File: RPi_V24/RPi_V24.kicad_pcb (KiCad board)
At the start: 4 copper layers, 65 x 56 mm, 65 parts, among them J1 DB9_Male, J10 Conn_01x03, J11 Conn_01x03, J12 Conn_01x03_Female, J13 Conn_02x04_Odd_Even, J14 Conn_01x03, J15 Conn_01x03, J16 Conn_02x05_Odd_Even, J17 Conn_02x05_Odd_Even, J18 Conn_02x05_Odd_Even, J2 DB9_Male, J3 40HAT, J4 DB9_Male, J5 Conn_02x04_Odd_Even, J6 Conn_01x03, J7 Conn_01x03, J8 Conn_02x04_Odd_Even, J9 CONN_01X02, U1 MAX561, U2 CAT24C32, U3 MAX561

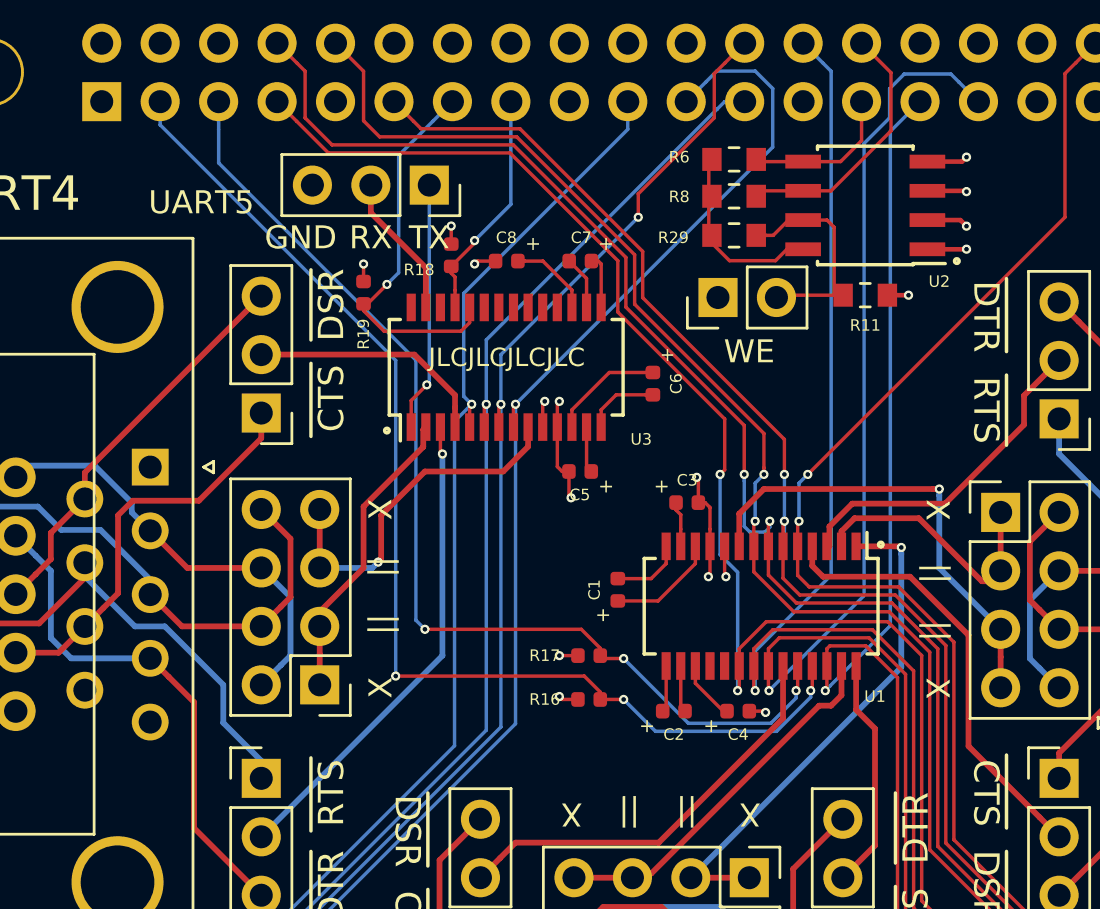
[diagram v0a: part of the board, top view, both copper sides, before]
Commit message: Silk screen adjustments.
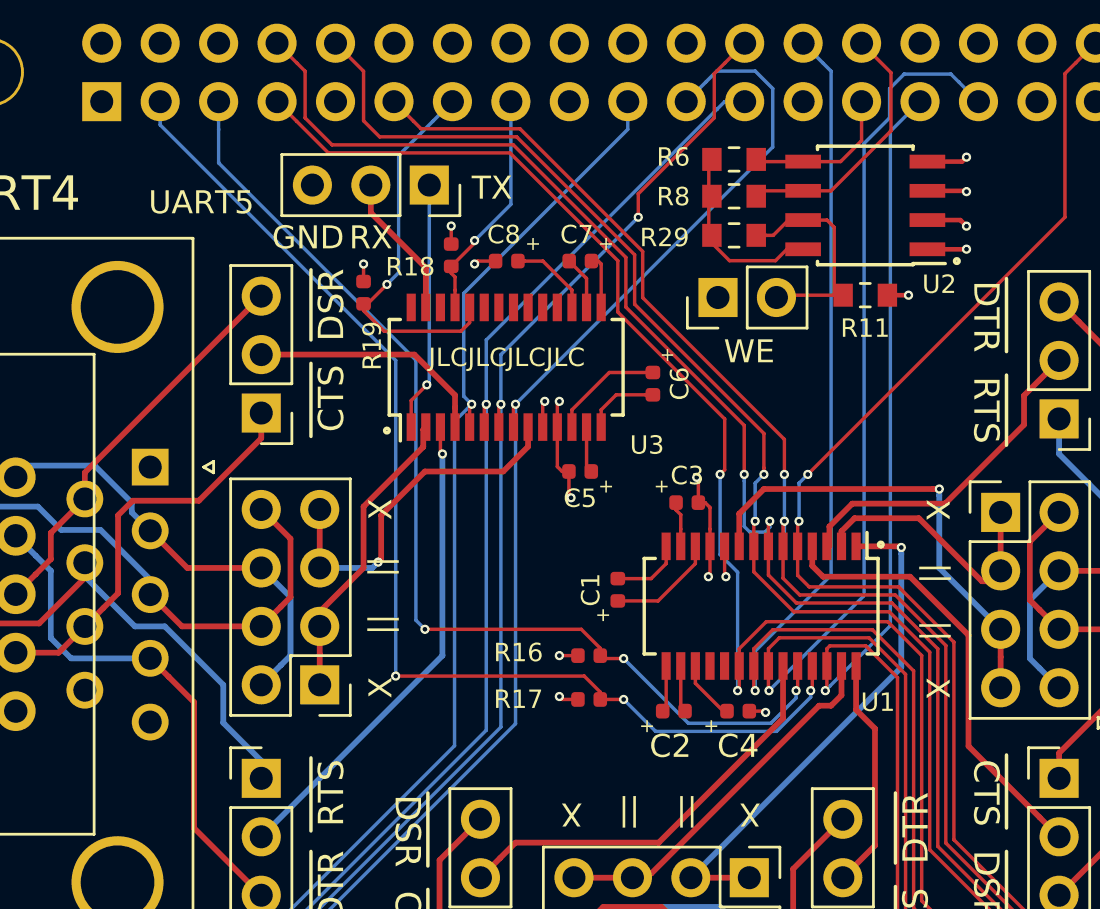
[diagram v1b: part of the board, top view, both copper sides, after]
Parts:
- R17, R19: value 0R -> 10K
